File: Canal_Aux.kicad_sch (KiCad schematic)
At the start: 0 parts

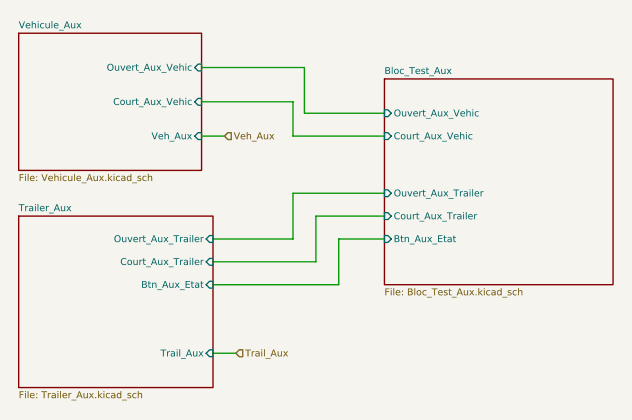
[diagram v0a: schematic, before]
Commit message: Add files via upload
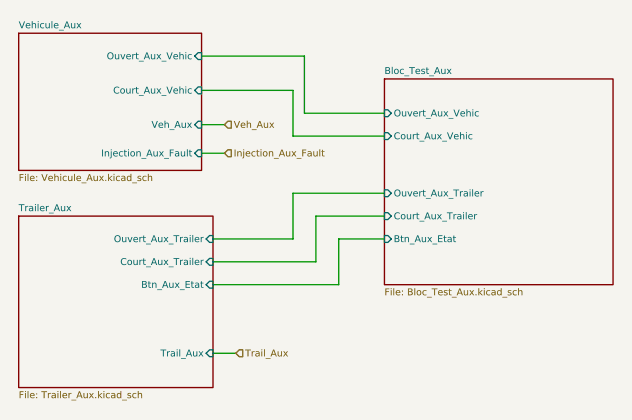
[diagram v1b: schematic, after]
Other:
- sheet Vehicule_Aux ports: added Injection_Aux_Fault; removed none
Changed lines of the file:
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@@
 	(wire
 		(pts
-			(xy 38.1 30.48) (xy 40.64 30.48)
+			(xy 38.1 29.21) (xy 40.64 29.21)
 		)
 		(stroke
@@
 	(wire
 		(pts
-			(xy 48.26 26.67) (xy 48.26 30.48)
+			(xy 48.26 25.4) (xy 48.26 30.48)
 		)
 		(stroke
@@
 	(wire
 		(pts
-			(xy 38.1 22.86) (xy 49.53 22.86)
-		)
-		(stroke
-			(width 0)
-			(type default)
-		)
-	)
-	(wire
-		(pts
-			(xy 38.1 26.67) (xy 48.26 26.67)
+			(xy 38.1 21.59) (xy 49.53 21.59)
+		)
+		(stroke
+			(width 0)
+			(type default)
+		)
+	)
+	(wire
+		(pts
+			(xy 38.1 25.4) (xy 48.26 25.4)
 		)
 		(stroke
@@
 	(wire
 		(pts
-			(xy 49.53 22.86) (xy 49.53 27.94)
+			(xy 49.53 21.59) (xy 49.53 27.94)
 		)
 		(stroke
@@
 		(pts
 			(xy 39.37 44.45) (xy 50.8 44.45)
+		)
+		(stroke
+			(width 0)
+			(type default)
+		)
+	)
+	(wire
+		(pts
+			(xy 38.1 32.385) (xy 40.64 32.385)
 		)
 		(stroke
@@
 	(hierarchical_label "Veh_Aux"
 		(shape input)
-		(at 40.64 30.48 0)
+		(at 40.64 29.21 0)
 		(effects
 			(font
@@
 		(shape input)
 		(at 41.91 54.61 0)
+		(effects
+			(font
+				(size 0.762 0.762)
+			)
+			(justify left)
+		)
+	)
+	(hierarchical_label "Injection_Aux_Fault"
+		(shape input)
+		(at 40.64 32.385 0)
 		(effects
 			(font
@@
 		)
 		(pin "Court_Aux_Vehic" input
-			(at 38.1 26.67 0)
+			(at 38.1 25.4 0)
 			(effects
 				(font
@@
 		)
 		(pin "Veh_Aux" input
-			(at 38.1 30.48 0)
+			(at 38.1 29.21 0)
 			(effects
 				(font
@@
 		)
 		(pin "Ouvert_Aux_Vehic" input
-			(at 38.1 22.86 0)
-			(effects
-				(font
+			(at 38.1 21.59 0)
+			(effects
+				(font
+					(size 0.762 0.762)
+				)
+				(justify right)
+			)
+		)
+		(pin "Injection_Aux_Fault" input
+			(at 38.1 32.385 0)
+			(effects
+				(font

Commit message: Add files via upload
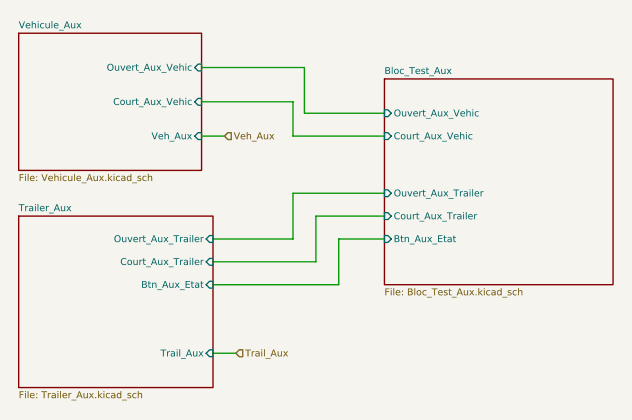
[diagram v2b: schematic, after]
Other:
- sheet Vehicule_Aux ports: added none; removed Injection_Aux_Fault
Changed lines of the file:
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@@
 	(wire
 		(pts
-			(xy 38.1 29.21) (xy 40.64 29.21)
+			(xy 38.1 30.48) (xy 40.64 30.48)
 		)
 		(stroke
@@
 	(wire
 		(pts
-			(xy 48.26 25.4) (xy 48.26 30.48)
+			(xy 48.26 26.67) (xy 48.26 30.48)
 		)
 		(stroke
@@
 	(wire
 		(pts
-			(xy 38.1 21.59) (xy 49.53 21.59)
-		)
-		(stroke
-			(width 0)
-			(type default)
-		)
-	)
-	(wire
-		(pts
-			(xy 38.1 25.4) (xy 48.26 25.4)
+			(xy 38.1 22.86) (xy 49.53 22.86)
+		)
+		(stroke
+			(width 0)
+			(type default)
+		)
+	)
+	(wire
+		(pts
+			(xy 38.1 26.67) (xy 48.26 26.67)
 		)
 		(stroke
@@
 	(wire
 		(pts
-			(xy 49.53 21.59) (xy 49.53 27.94)
+			(xy 49.53 22.86) (xy 49.53 27.94)
 		)
 		(stroke
@@
 		(pts
 			(xy 39.37 44.45) (xy 50.8 44.45)
-		)
-		(stroke
-			(width 0)
-			(type default)
-		)
-	)
-	(wire
-		(pts
-			(xy 38.1 32.385) (xy 40.64 32.385)
 		)
 		(stroke
@@
 	(hierarchical_label "Veh_Aux"
 		(shape input)
-		(at 40.64 29.21 0)
+		(at 40.64 30.48 0)
 		(effects
 			(font
@@
 		(shape input)
 		(at 41.91 54.61 0)
-		(effects
-			(font
-				(size 0.762 0.762)
-			)
-			(justify left)
-		)
-	)
-	(hierarchical_label "Injection_Aux_Fault"
-		(shape input)
-		(at 40.64 32.385 0)
 		(effects
 			(font
@@
 		)
 		(pin "Court_Aux_Vehic" input
-			(at 38.1 25.4 0)
+			(at 38.1 26.67 0)
 			(effects
 				(font
@@
 		)
 		(pin "Veh_Aux" input
-			(at 38.1 29.21 0)
+			(at 38.1 30.48 0)
 			(effects
 				(font
@@
 		)
 		(pin "Ouvert_Aux_Vehic" input
-			(at 38.1 21.59 0)
-			(effects
-				(font
-					(size 0.762 0.762)
-				)
-				(justify right)
-			)
-		)
-		(pin "Injection_Aux_Fault" input
-			(at 38.1 32.385 0)
-			(effects
-				(font
+			(at 38.1 22.86 0)
+			(effects
+				(font
